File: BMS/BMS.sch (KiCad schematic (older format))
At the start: 76 parts, among them J1 Cell Taps, J2 IsoSPI, J3 Temp 1, J4 Temp 2, J5 Temp 3, J6 Temp 4, J7 Temp 5, J8 Temp 6, J9 Temp 7, Q1 NSV1C201MZ4, Q2 BSS308PE, Q3 BSS308PE, Q4 BSS308PE, Q5 BSS308PE, Q6 BSS308PE, Q7 BSS308PE, Q8 BSS308PE, SW1 SW_DIP_x04, U1 LTC6811, U2 ADG708

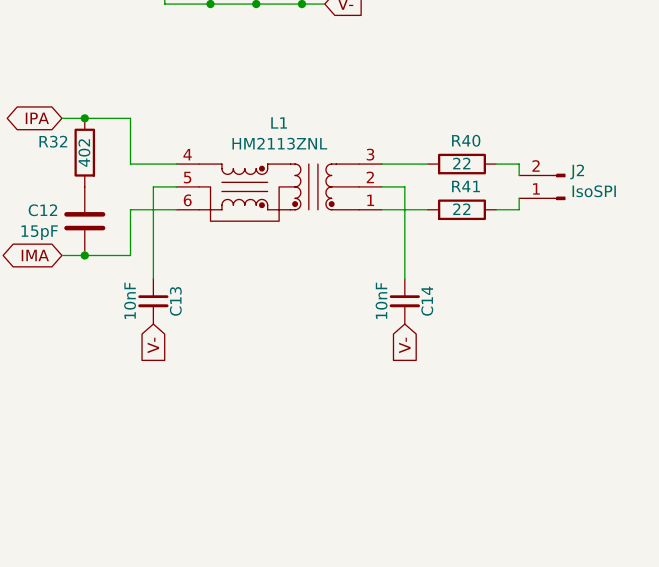
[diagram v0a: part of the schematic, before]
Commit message: yikes
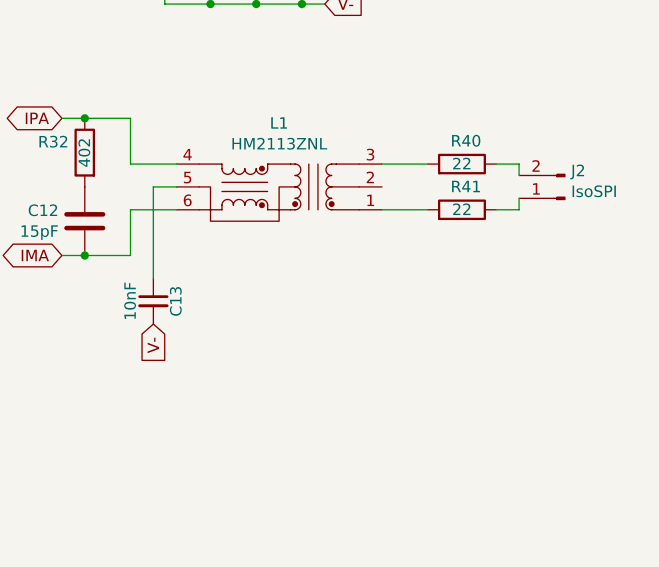
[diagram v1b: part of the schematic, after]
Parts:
- removed C14: 10nF, Capacitors_SMD:C_0805_HandSoldering, symbol Device:C_Small
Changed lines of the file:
@@
 Wire Wire Line
 	9250 2550 9350 2550
-$Comp
-L Device:R R40
-U 1 1 5CA16E1A
-P 10600 2450
-F 0 "R40" V 10700 2400 50  0000 L CNN
-F 1 "22" V 10600 2450 50  0000 C CNN
-F 2 "Resistors_SMD:R_0805_HandSoldering" V 10530 2450 50  0001 C CNN
-F 3 "~" H 10600 2450 50  0001 C CNN
-	1    10600 2450
-	0    1    -1   0
-$EndComp
-$Comp
-L Device:R R41
-U 1 1 5CA1723F
-P 10600 2650
-F 0 "R41" V 10700 2600 50  0000 L CNN
-F 1 "22" V 10600 2650 50  0000 C CNN
-F 2 "Resistors_SMD:R_0805_HandSoldering" V 10530 2650 50  0001 C CNN
-F 3 "~" H 10600 2650 50  0001 C CNN
-	1    10600 2650
-	0    1    -1   0
-$EndComp
 Wire Wire Line
 	10750 2450 10850 2450
@@
 Wire Wire Line
 	10850 2650 10750 2650
-$Comp
-L Device:C_Small C14
-U 1 1 5CA52F72
-P 10350 3050
-F 0 "C14" V 10450 3050 50  0000 C CNN
-F 1 "10nF" V 10250 3050 50  0000 C CNN
-F 2 "Capacitors_SMD:C_0805_HandSoldering" H 10388 2900 50  0001 C CNN
-F 3 "~" H 10350 3050 50  0001 C CNN
-	1    10350 3050
-	1    0    0    -1
-$EndComp
-Text GLabel 10350 3150 3    50   Input ~ 0
-V-
-Wire Wire Line
-	10350 2950 10350 2550
-Wire Wire Line
-	10250 2550 10350 2550
 Wire Wire Line
 	10250 2450 10450 2450
@@
 Text GLabel 8350 850  2    50   Output ~ 0
 VREG
+$Comp
+L Device:R R41
+U 1 1 5CA1723F
+P 10600 2650
+F 0 "R41" V 10700 2600 50  0000 L CNN
+F 1 "22" V 10600 2650 50  0000 C CNN
+F 2 "Resistors_SMD:R_0805_HandSoldering" V 10530 2650 50  0001 C CNN
+F 3 "~" H 10600 2650 50  0001 C CNN
+	1    10600 2650
+	0    1    -1   0
+$EndComp
+$Comp
+L Device:R R40
+U 1 1 5CA16E1A
+P 10600 2450
+F 0 "R40" V 10700 2400 50  0000 L CNN
+F 1 "22" V 10600 2450 50  0000 C CNN
+F 2 "Resistors_SMD:R_0805_HandSoldering" V 10530 2450 50  0001 C CNN
+F 3 "~" H 10600 2450 50  0001 C CNN
+	1    10600 2450
+	0    1    -1   0
+$EndComp
 $EndSCHEMATC
